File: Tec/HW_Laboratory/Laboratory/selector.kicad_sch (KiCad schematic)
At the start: 2 parts, among them J1 ENTRADA, J2 SALIDA

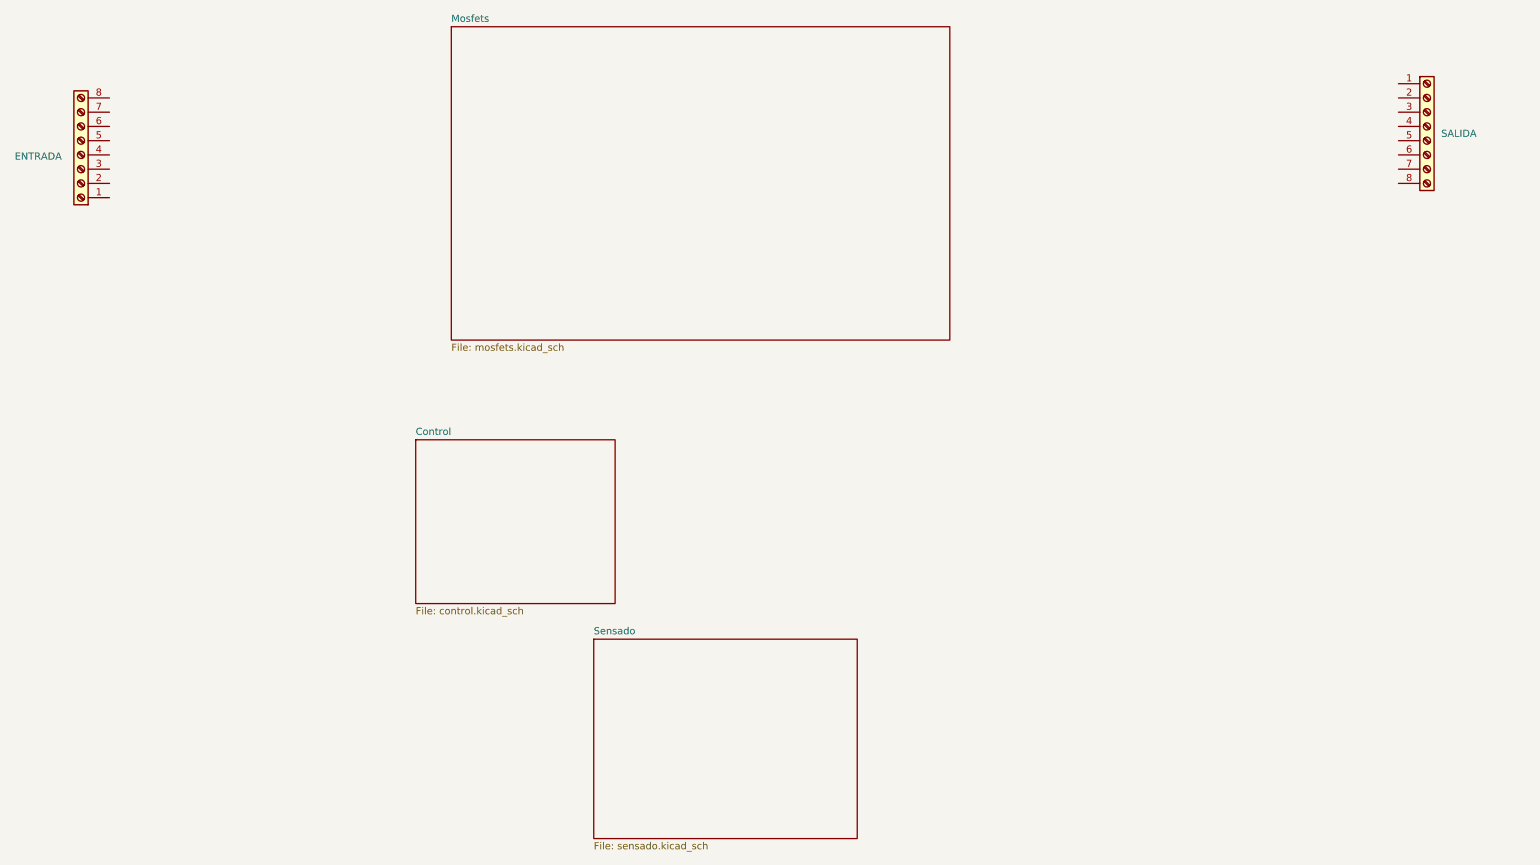
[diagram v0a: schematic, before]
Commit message: Schematics UPDATE
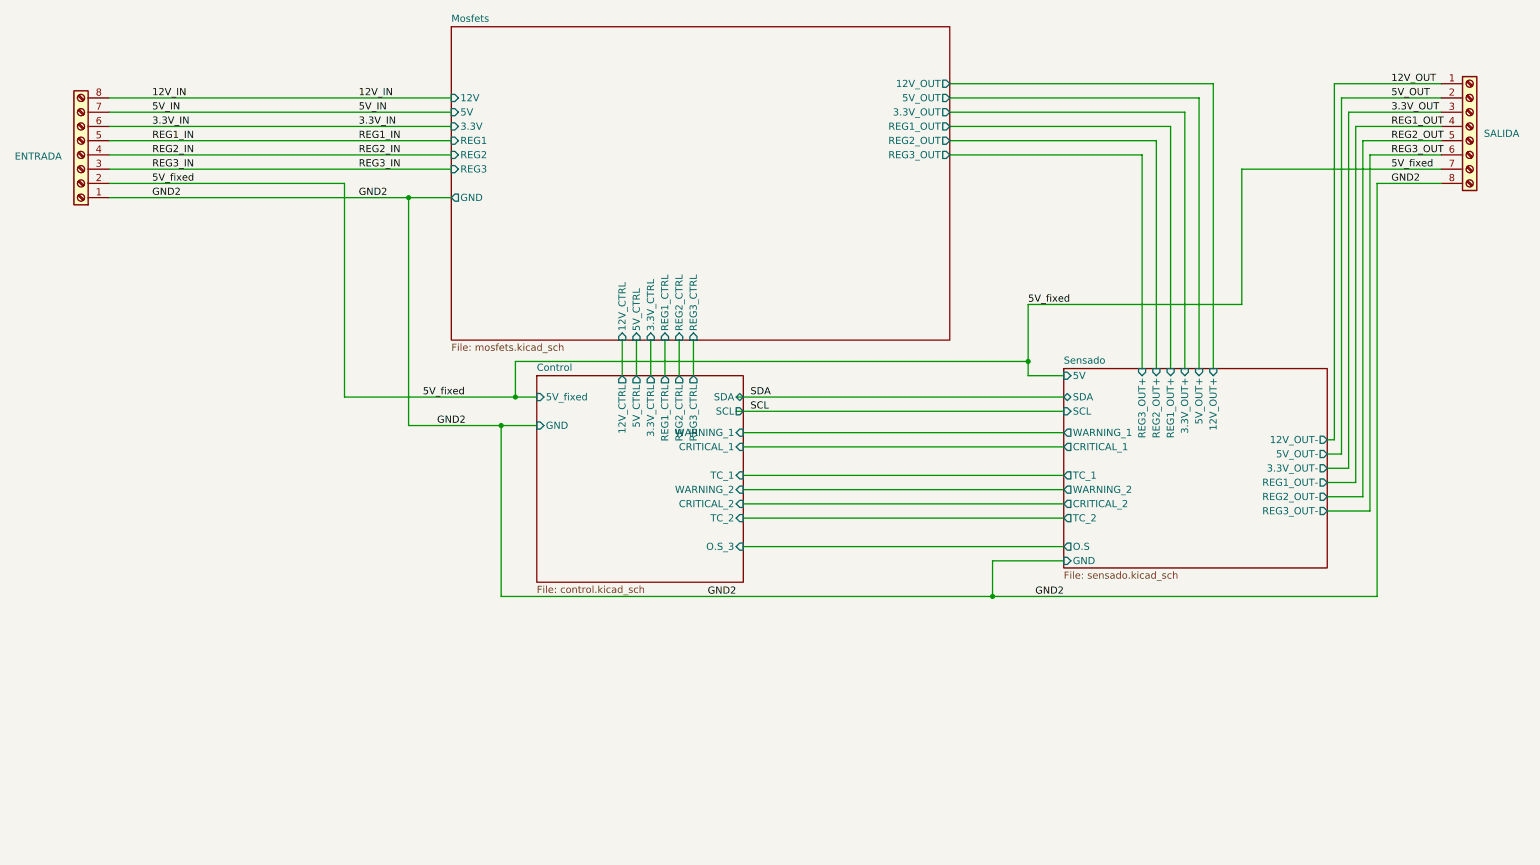
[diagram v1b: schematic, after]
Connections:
- net 12V_OUT: now reaches J2.1 (Pin_1)
- net 5V_OUT: now reaches J2.2 (Pin_2)
- net 3.3V_OUT: now reaches J2.3 (Pin_3)
- net REG1_OUT: now reaches J2.4 (Pin_4)
- net REG2_OUT: now reaches J2.5 (Pin_5)
- net REG3_OUT: now reaches J2.6 (Pin_6)
- net 5V_fixed: now reaches J2.7 (Pin_7)
- net 5V_fixed: now also J1.2 (Pin_2)
- net GND2: now reaches J2.8 (Pin_8)
- net GND2: now also J1.1 (Pin_1)
- net REG3_IN: now reaches J1.3 (Pin_3)
- net REG2_IN: now reaches J1.4 (Pin_4)
- net REG1_IN: now reaches J1.5 (Pin_5)
- net 3.3V_IN: now reaches J1.6 (Pin_6)
- net 5V_IN: now reaches J1.7 (Pin_7)
- net 12V_IN: now reaches J1.8 (Pin_8)
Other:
- sheet Control ports: added 12V_CTRL, 3.3V_CTRL, 5V_CTRL, 5V_fixed, CRITICAL_1, CRITICAL_2, GND, O.S_3, REG1_CTRL, REG2_CTRL, REG3_CTRL, SCL, SDA, TC_1, TC_2, WARNING_1, WARNING_2; removed none
- sheet Mosfets ports: added 12V, 12V_CTRL, 12V_OUT, 3.3V, 3.3V_CTRL, 3.3V_OUT, 5V, 5V_CTRL, 5V_OUT, GND, REG1, REG1_CTRL, REG1_OUT, REG2, REG2_CTRL, REG2_OUT, REG3, REG3_CTRL, REG3_OUT; removed none
- sheet Sensado ports: added 12V_OUT+, 12V_OUT-, 3.3V_OUT+, 3.3V_OUT-, 5V, 5V_OUT+, 5V_OUT-, CRITICAL_1, CRITICAL_2, GND, O.S, REG1_OUT+, REG1_OUT-, REG2_OUT+, REG2_OUT-, REG3_OUT+, REG3_OUT-, SCL, SDA, TC_1, TC_2, WARNING_1, WARNING_2; removed none
